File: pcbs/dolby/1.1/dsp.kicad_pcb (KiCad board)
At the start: 2 copper layers, 85 x 55 mm, 74 parts, among them J1 Conn_01x04_Pin, J2 Conn_01x04_Pin, J3 Conn_01x02, J4 Conn_01x02_Pin, J5 Conn_01x03_Pin, J6 Conn_01x04_Male, J7 Conn_01x02, U1 TLV1117LV-25, U2 AZ1117CH2-3.3, U3 DA101C_C6931652, U4 SPA130, U5 TLV1117LV-25, U6 TMP100, X1 ECS-3225SMV-270-FP-TR

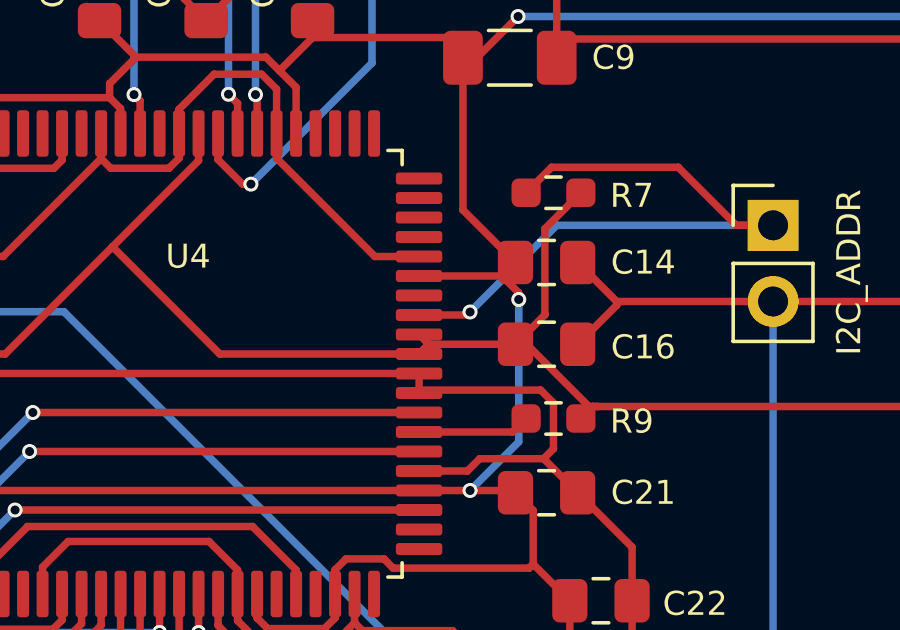
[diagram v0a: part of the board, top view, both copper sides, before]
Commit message: UPdates
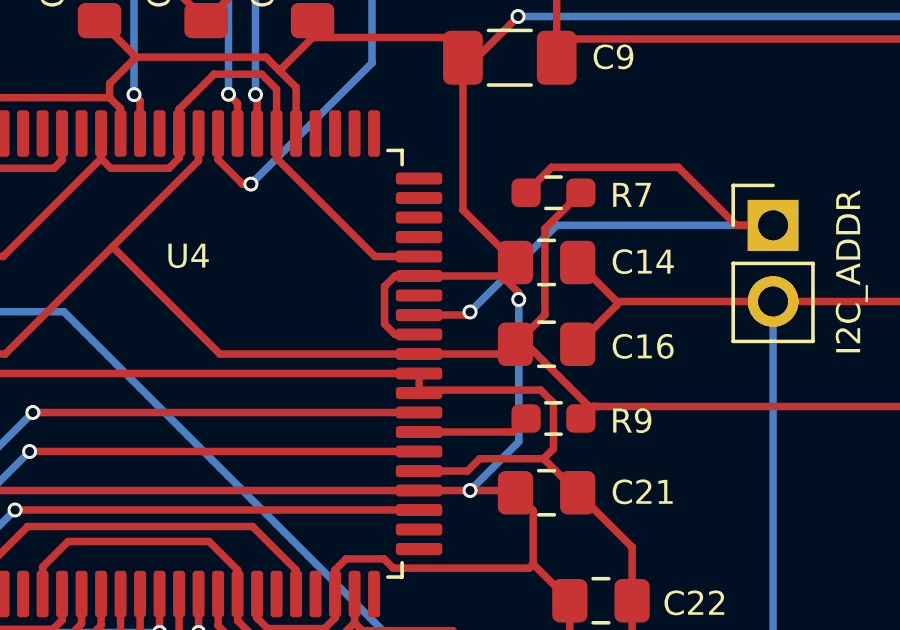
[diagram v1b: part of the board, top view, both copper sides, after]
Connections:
- U4 pad 52: 3V3 -> 2.5V
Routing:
- net 2.5V: track 180.1 -> 184.0 mm
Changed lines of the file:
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@@
 			(layers "F.Cu" "F.Mask" "F.Paste")
 			(roundrect_rratio 0.25)
-			(net 1 "3V3")
+			(net 8 "2.5V")
 			(pinfunction "TESTB")
 			(pintype "input")
@@
 	)
 	(segment
-		(start 75.3489 55.59)
-		(end 72.4614 55.59)
-		(width 0.25)
-		(layer "F.Cu")
-		(net 1)
-	)
-	(segment
 		(start 76.1739 40.465)
 		(end 102.486 40.465)
@@
 	)
 	(segment
+		(start 72.1364 55.915)
+		(end 75.0239 55.915)
+		(width 0.25)
+		(layer "F.Cu")
+		(net 1)
+	)
+	(segment
 		(start 71.9835 66.1895)
 		(end 66.6609 66.1895)
@@
 	)
 	(segment
-		(start 72.2987 55.7527)
-		(end 72.1364 55.915)
+		(start 75.0239 55.915)
+		(end 75.3489 55.59)
 		(width 0.25)
 		(layer "F.Cu")
@@
 	)
 	(segment
-		(start 72.1364 55.265)
-		(end 72.4614 55.59)
-		(width 0.25)
-		(layer "F.Cu")
-		(net 1)
-	)
-	(segment
 		(start 93.4364 74.5025)
 		(end 93.4364 75.165)
@@
 	)
 	(segment
-		(start 72.4614 55.59)
-		(end 72.2987 55.7527)
-		(width 0.25)
-		(layer "F.Cu")
-		(net 1)
-	)
-	(segment
 		(start 58.0934 43.8373)
 		(end 64.0712 43.8373)
@@
 	)
 	(segment
+		(start 71.335462 55.265)
+		(end 70.9854 54.914938)
+		(width 0.25)
+		(layer "F.Cu")
+		(net 8)
+	)
+	(segment
 		(start 68.9827 65.0684)
 		(end 67.0901 65.0684)
@@
 	)
 	(segment
+		(start 71.335462 53.315)
+		(end 72.1364 53.315)
+		(width 0.25)
+		(layer "F.Cu")
+		(net 8)
+	)
+	(segment
 		(start 62.7035 46.0196)
 		(end 61.4864 44.8025)
@@
 	)
 	(segment
+		(start 70.9854 54.914938)
+		(end 70.9854 53.665062)
+		(width 0.25)
+		(layer "F.Cu")
+		(net 8)
+	)
+	(segment
 		(start 68.5864 45.3671)
 		(end 73.3179 45.3671)
@@
 	)
 	(segment
+		(start 70.9854 53.665062)
+		(end 71.335462 53.315)
+		(width 0.25)
+		(layer "F.Cu")
+		(net 8)
+	)
+	(segment
 		(start 66.7364 64.7147)
 		(end 66.7364 63.915)
@@
 		(width 0.25)
 		(layer "F.Cu")
+		(net 8)
+	)
+	(segment
+		(start 72.1364 55.265)
+		(end 71.335462 55.265)
+		(width 0.25)
+		(layer "F.Cu")
